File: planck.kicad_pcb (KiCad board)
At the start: 4 copper layers, 76.6 x 75.1 mm, 32 parts, among them J1 USB_C_Receptacle_USB2.0, K1 KEYSW, K2 KEYSW, K3 KEYSW, K4 KEYSW, SW1 SW_PUSH, U1 ATmega32U4-M, Y1 Crystal_GND24_Small

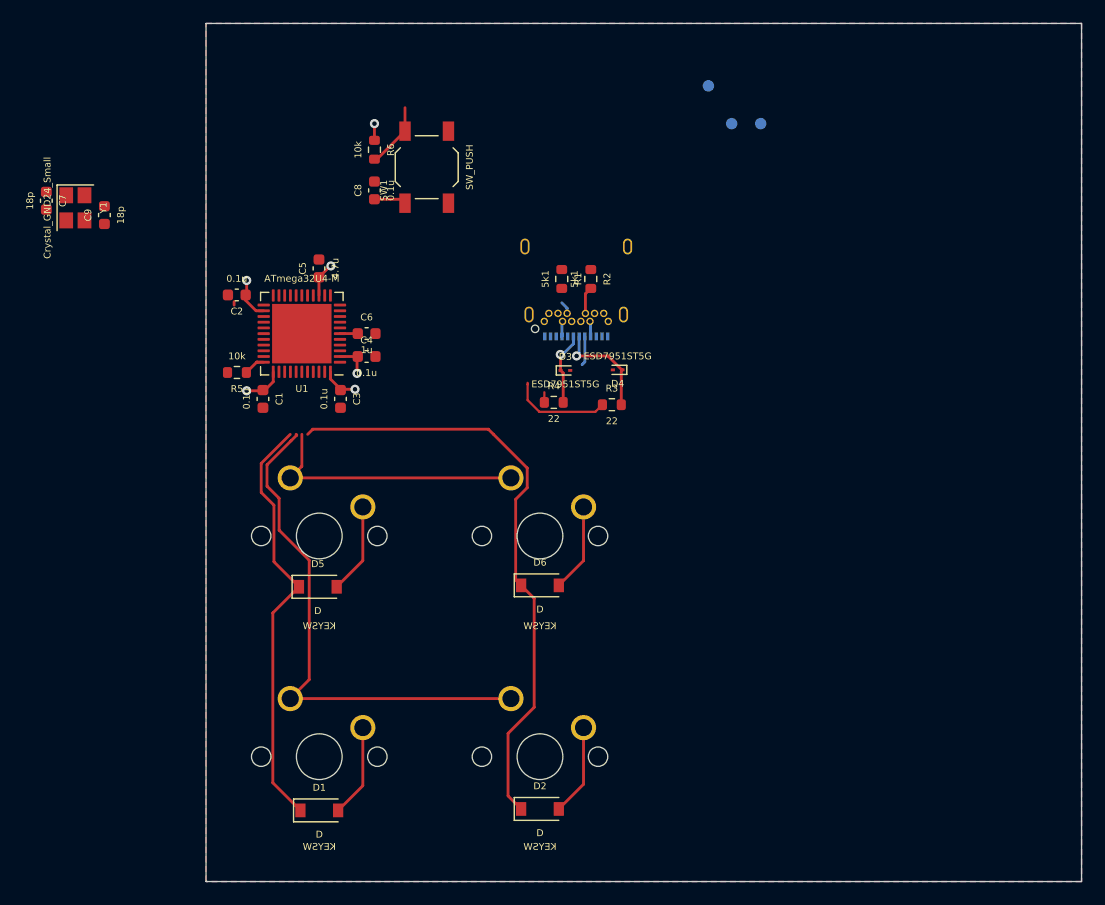
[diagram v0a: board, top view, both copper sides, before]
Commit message: finished layout
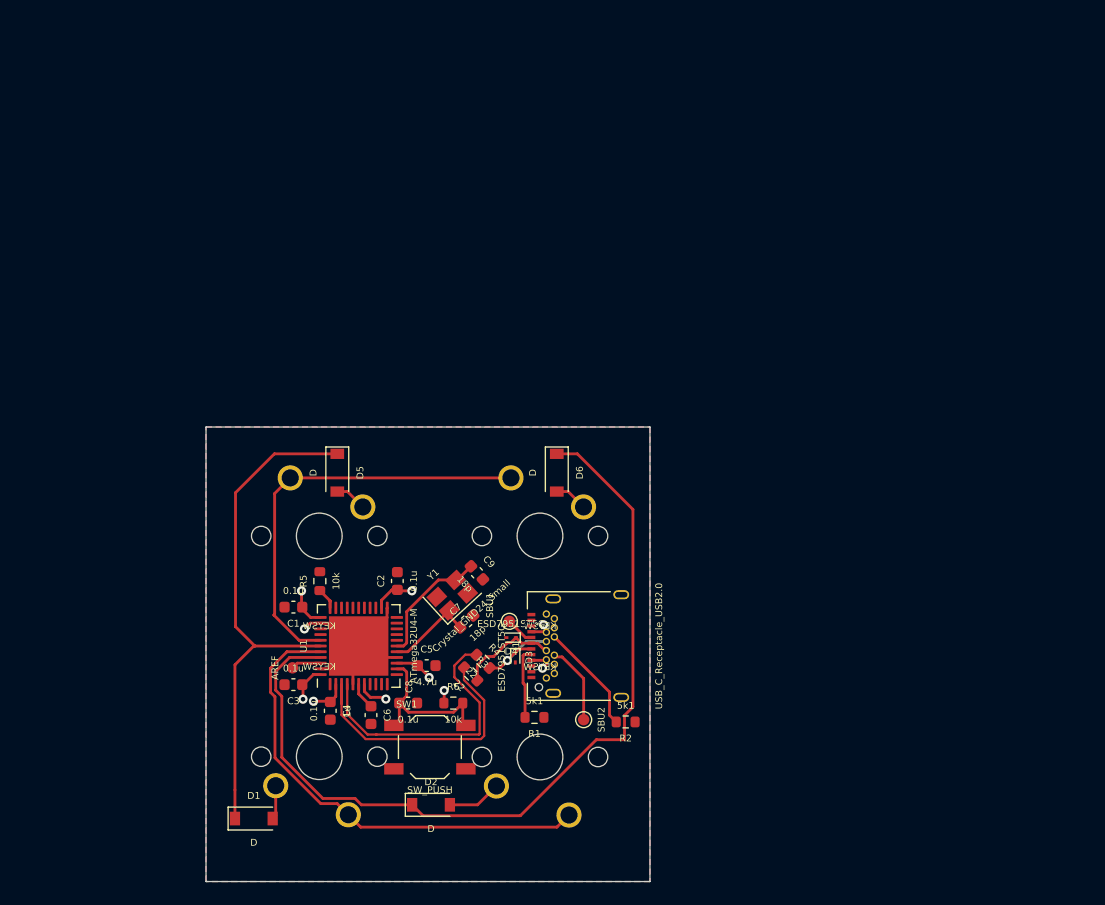
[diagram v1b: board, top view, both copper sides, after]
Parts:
- J1, TP1, TP2: moved to F.Cu
- moved TP3 62.6 mm to (85.0, 118.5), turned to 180 degrees
- moved TP2 54.4 mm to (110.5, 123.0), turned to 90 degrees
- moved C7 52.0 mm to (100.3, 114.4), turned to 42.5 degrees
- moved SW1 50.7 mm to (97.0, 125.4), turned to 0 degrees
- moved R6 48.9 mm to (99.1, 121.6), turned to 0 degrees
- moved TP1 47.7 mm to (104.0, 114.4), turned to -90 degrees
- moved Y1 47.3 mm to (99.0, 112.1), turned to 42.5 degrees
- moved C9 45.2 mm to (101.2, 110.2), turned to -47.5 degrees
- moved C8 44.9 mm to (95.2, 121.6), turned to 0 degrees
- moved R2 38.9 mm to (114.2, 123.2), turned to 180 degrees
- moved R1 38.4 mm to (106.2, 122.8), turned to 180 degrees
- moved C5 36.0 mm to (96.8, 118.3), turned to 0 degrees
- moved C6 33.4 mm to (91.9, 122.6), turned to -90 degrees
- moved J1 32.1 mm to (110.9, 116.6), turned to 90 degrees
- moved C4 31.2 mm to (88.3, 122.2), turned to -90 degrees
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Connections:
- U1 pad 38: /row0 -> /col1
- U1 pad 39: /col0 -> /row0
- U1 pad 40: /col1 -> /col0
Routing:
- net /D+: track 0.89 -> 24.2 mm
- net /row1: track 53.1 -> 76.1 mm
- net GND: track 0.30 -> 21.6 mm, vias 0 -> 1
- net /D-: track 8.74 -> 24.6 mm
- net /col1: track 24.3 -> 36.9 mm
- net /XTAL1: track 0.00 -> 11.4 mm
- net /row0: track 37.3 -> 46.0 mm
- net /XTAL2: track 0.00 -> 7.94 mm
- net Net-(J1-PadB5): track 2.38 -> 9.68 mm
- net /~reset: track 7.85 -> 14.4 mm
- net Net-(J1-PadA5): track 0.00 -> 6.24 mm
- net Net-(J1-PadB8): track 1.12 -> 7.01 mm
- net Net-(D1-Pad2): track 8.13 -> 2.98 mm
- net Net-(D5-Pad2): track 7.93 -> 2.79 mm
- net Net-(D6-Pad2): track 7.80 -> 2.90 mm
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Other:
- board size 76.6 x 75.1 mm -> 38.8 x 39.8 mm
